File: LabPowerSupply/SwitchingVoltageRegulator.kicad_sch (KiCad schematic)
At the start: 14 parts

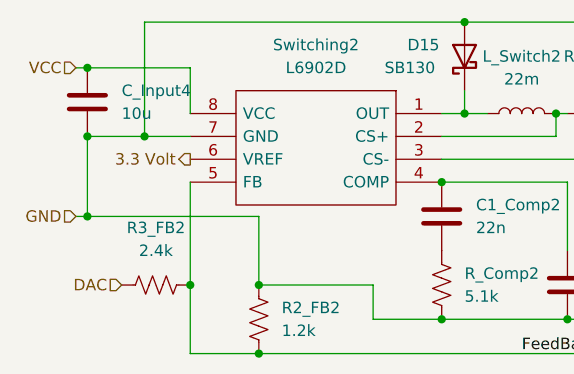
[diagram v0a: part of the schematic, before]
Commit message: started PCB
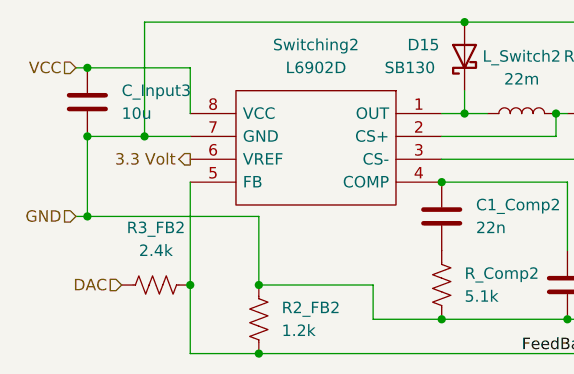
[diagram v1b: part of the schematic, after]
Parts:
- L_Switch2: footprint Inductor_THT:L_Radial_D8.7mm_P5.00mm_Fastron_07HCP -> Inductor_THT:L_Radial_D6.0mm_P4.00mm
- Switching2: footprint (none) -> Package_SO:SOIC-8-1EP_3.9x4.9mm_P1.27mm_EP2.95x4.9mm_Mask2.71x3.4mm
- renumbered C_Input4 to C_Input3
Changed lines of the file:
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@@
     (property "Reference" "Switching2" (id 0) (at 124.46 85.09 0))
     (property "Value" "L6902D" (id 1) (at 124.46 87.63 0))
-    (property "Footprint" "" (id 2) (at 114.3 90.17 0)
+    (property "Footprint" "Package_SO:SOIC-8-1EP_3.9x4.9mm_P1.27mm_EP2.95x4.9mm_Mask2.71x3.4mm" (id 2) (at 114.3 90.17 0)
       (effects (font (size 1.27 1.27)) (justify left) hide)
     )
@@
     (property "Reference" "L_Switch2" (id 0) (at 147.32 86.36 90))
     (property "Value" "22m" (id 1) (at 147.32 88.9 90))
-    (property "Footprint" "Inductor_THT:L_Radial_D8.7mm_P5.00mm_Fastron_07HCP" (id 2) (at 147.32 92.71 0)
+    (property "Footprint" "Inductor_THT:L_Radial_D6.0mm_P4.00mm" (id 2) (at 147.32 92.71 0)
       (effects (font (size 1.27 1.27)) hide)
     )
@@
   (symbol (lib_id "Device:C") (at 99.06 91.44 0) (unit 1)
     (in_bom yes) (on_board yes) (fields_autoplaced)
-    (property "Reference" "C_Input4" (id 0) (at 102.87 90.1699 0)
+    (property "Reference" "C_Input3" (id 0) (at 102.87 90.1699 0)
       (effects (font (size 1.27 1.27)) (justify left))
     )

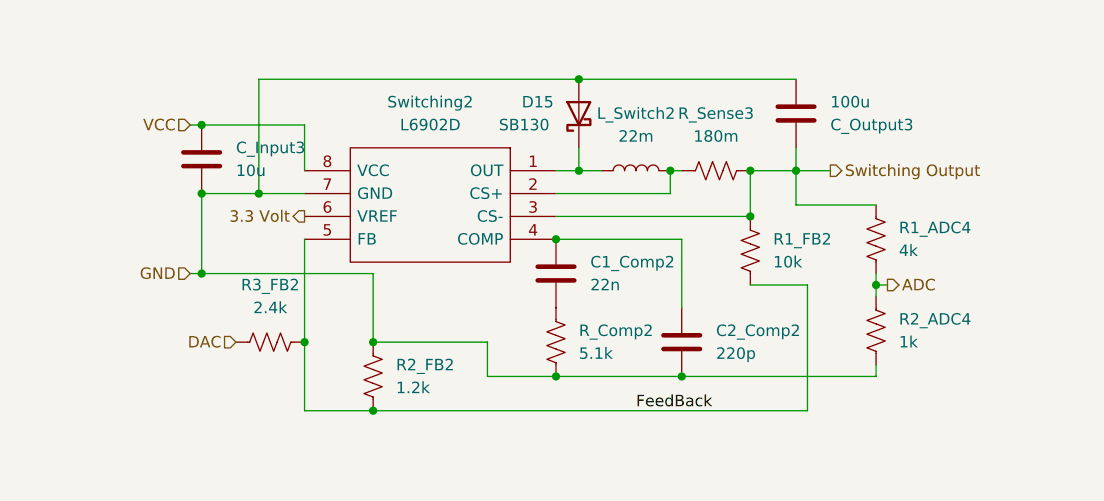
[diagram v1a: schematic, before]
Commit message: more work
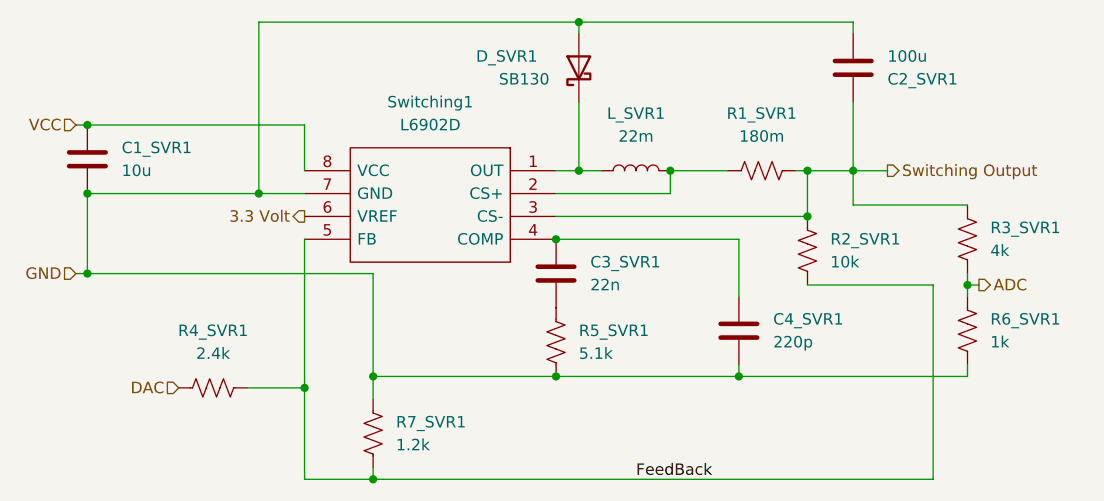
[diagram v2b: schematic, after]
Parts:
- renumbered C_Input3 to C1_SVR1, C_Output3 to C2_SVR1, C1_Comp2 to C3_SVR1, C2_Comp2 to C4_SVR1, D15 to D_SVR1, L_Switch2 to L_SVR1, R_Sense3 to R1_SVR1, R1_FB2 to R2_SVR1, R1_ADC4 to R3_SVR1, R3_FB2 to R4_SVR1, R_Comp2 to R5_SVR1, R2_ADC4 to R6_SVR1, R2_FB2 to R7_SVR1, Switching2 to Switching1
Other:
- moved on the sheet: C1_SVR1, C2_SVR1, C4_SVR1, D_SVR1, R1_SVR1, R2_SVR1, R3_SVR1, R4_SVR1, R6_SVR1, R7_SVR1
